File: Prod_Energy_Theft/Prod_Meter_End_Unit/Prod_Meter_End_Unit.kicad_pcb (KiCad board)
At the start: 4 copper layers, 150.7 x 71.9 mm, 83 parts, among them J1 Screw_Terminal_01x02, J15 Screw_Terminal_01x01, J16 Screw_Terminal_01x01, J17 Screw_Terminal_01x01, J18 Screw_Terminal_01x01, J19 Screw_Terminal_01x01, J2 Screw_Terminal_01x02, J20 Screw_Terminal_01x01, J21 Screw_Terminal_01x01, J22 Screw_Terminal_01x01, J23 Screw_Terminal_01x01, J3 Screw_Terminal_01x02, J4 Conn_01x06_Pin, J5 Screw_Terminal_01x02, J6 Jack-DC, K1 TQ2-L2-5V, Q3 AO3400A, Q4 AO3400A, U2 ESP32-C6-MINI-1, U3 BD00FC0WEFJ, U5 ADE7816ACPZ, Y2 Crystal

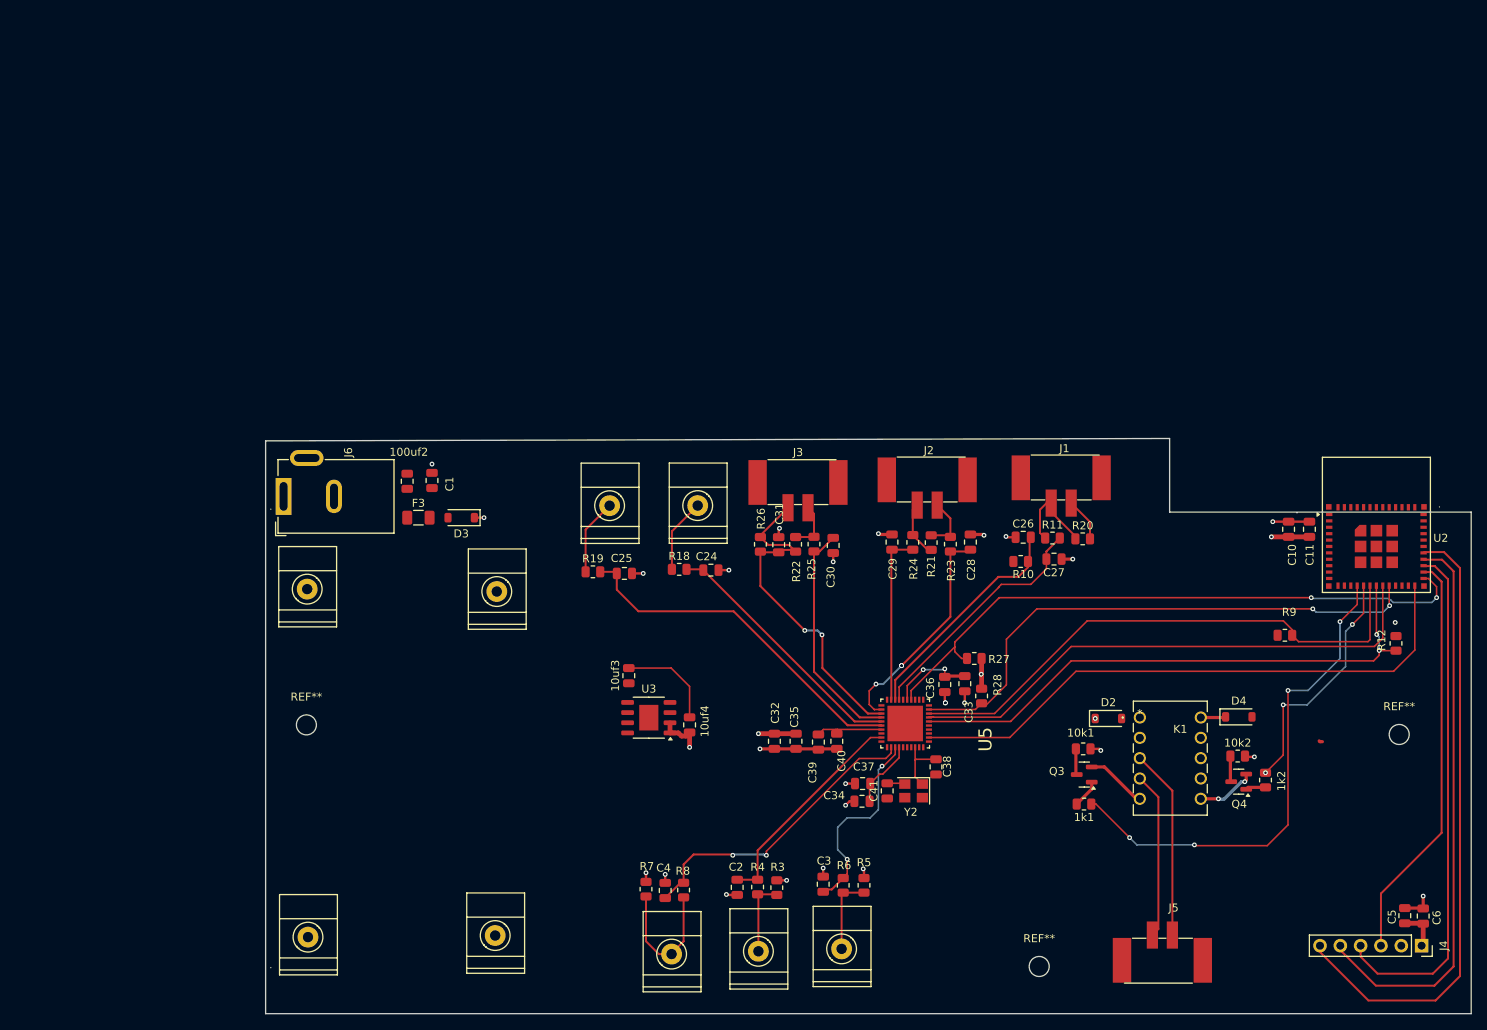
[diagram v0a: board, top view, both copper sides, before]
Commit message: PCB
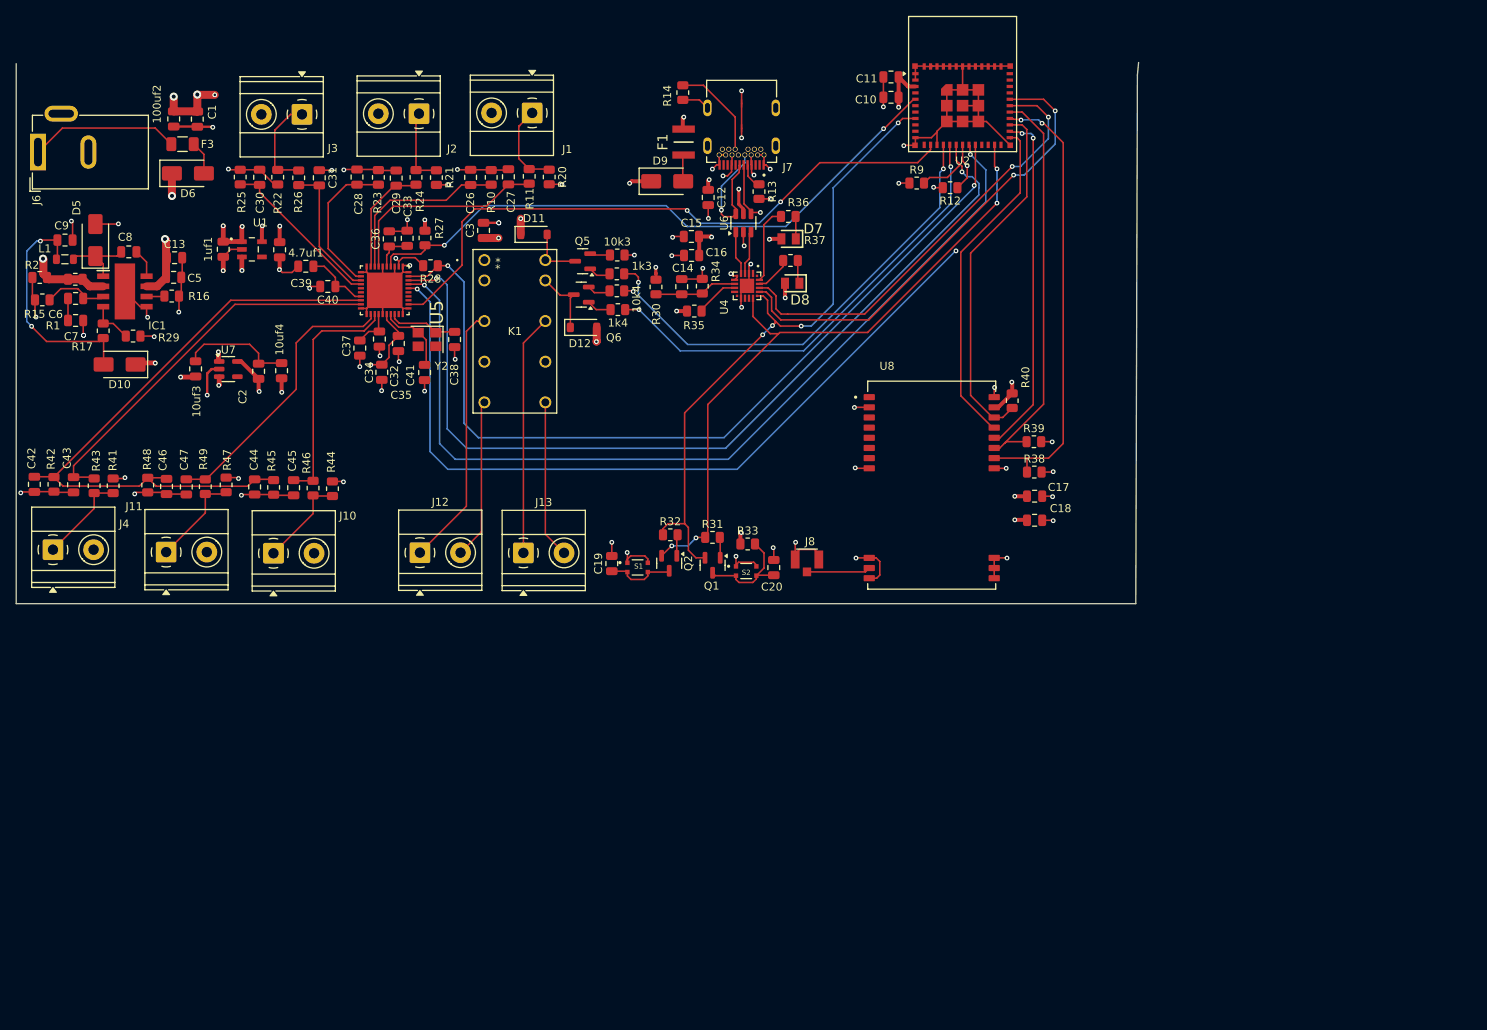
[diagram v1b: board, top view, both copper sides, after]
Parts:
- removed 10k1, 10k2, 1k1, 1k2, R3, R5, R7: R, Resistor_SMD:R_0805_2012Metric
- removed C24, C25, C4: 22nf, Capacitor_SMD:C_0805_2012Metric
- removed D2, D3, D4: D, Diode_SMD:D_SOD-123
- removed J15, J16, J17, J18, J19, J20, J21, J22, J23: Screw_Terminal_01x01, custom:TerminalBlock_1x01_P5.08mm
- removed J5: Screw_Terminal_01x02, TerminalBlock_Phoenix:TerminalBlock_Phoenix_PTSM-0,5-2-2,5-V-SMD_1x02-1MP_P2.50mm_Vertical
- removed Q3, Q4: AO3400A, Package_TO_SOT_SMD:SOT-23
- removed R18, R19: 10k, Resistor_SMD:R_0805_2012Metric
- removed R4, R6, R8: 1k, Resistor_SMD:R_0805_2012Metric
- removed REF** (x3): MountingHole_2.5mm, MountingHole:MountingHole_2.5mm
- removed U3: BD00FC0WEFJ, Package_SO:HTSOP-8-1EP_3.9x4.9mm_P1.27mm_EP2.4x3.2mm
- added 10k3: R, Resistor_SMD:R_0805_2012Metric, F.Cu at (134.8, 67.4)
- added 10k4: R, Resistor_SMD:R_0805_2012Metric, F.Cu at (134.7, 71.8)
- added 1k3: R, Resistor_SMD:R_0805_2012Metric, F.Cu at (134.7, 69.7)
- added 1k4: R, Resistor_SMD:R_0805_2012Metric, F.Cu at (134.8, 74.2)
- added 1uf1: C, Capacitor_SMD:C_0805_2012Metric, F.Cu at (85.5, 66.7)
- added 4.7uf1: C, Capacitor_SMD:C_0805_2012Metric, F.Cu at (92.6, 66.7)
- added C12: 0.1u, Capacitor_SMD:C_0805_2012Metric, F.Cu at (146.1, 60.2)
- added C13: 100nf, Capacitor_SMD:C_0805_2012Metric, F.Cu at (79.4, 67.7)
- added C14: 1u, Capacitor_SMD:C_0805_2012Metric, F.Cu at (142.8, 71.3)
- added C15: 4.7u, Capacitor_SMD:C_0805_2012Metric, F.Cu at (144.0, 65.0)
- added C16: 0.1u, Capacitor_SMD:C_0805_2012Metric, F.Cu at (144.1, 67.4)
- added C17: 10u, Capacitor_SMD:C_0805_2012Metric, F.Cu at (186.9, 97.5)
- added C18: 0.1u, Capacitor_SMD:C_0805_2012Metric, F.Cu at (186.9, 100.5)
- added C19: 0.1u, Capacitor_SMD:C_0805_2012Metric, F.Cu at (134.1, 105.9)
- added C20: 1u, Capacitor_SMD:C_0805_2012Metric, F.Cu at (154.3, 106.4)
- added C42: 22nf, Capacitor_SMD:C_0805_2012Metric, F.Cu at (61.9, 96.0)
- added C43: 22nf, Capacitor_SMD:C_0805_2012Metric, F.Cu at (66.8, 96.1)
- added C44: 22nf, Capacitor_SMD:C_0805_2012Metric, F.Cu at (89.4, 96.4)
- added C45: 22nf, Capacitor_SMD:C_0805_2012Metric, F.Cu at (94.3, 96.5)
- added C46: 22nf, Capacitor_SMD:C_0805_2012Metric, F.Cu at (78.4, 96.3)
- added C47: 22nf, Capacitor_SMD:C_0805_2012Metric, F.Cu at (80.9, 96.3)
- added C7: C, Capacitor_SMD:C_0805_2012Metric, F.Cu at (67.0, 75.5)
- added C8: 100nf, Capacitor_SMD:C_0805_2012Metric, F.Cu at (73.7, 67.0)
- added C9: 47uf, Capacitor_SMD:C_0805_2012Metric, F.Cu at (65.7, 65.5)
- added D10: SS34, Diode_SMD:D_SMA, F.Cu at (72.5, 81.0)
- added D11: D, Diode_SMD:D_SOD-123, F.Cu at (124.3, 64.8)
- added D12: D, Diode_SMD:D_SOD-123, F.Cu at (130.5, 76.4)
- added D5: SS34, Diode_SMD:D_SMA, F.Cu at (69.5, 65.5)
- added D6: SS34, Diode_SMD:D_SMA, F.Cu at (81.1, 57.2)
- added D7: Green, theftdetection:LEDC2012X120N, F.Cu at (156.2, 65.3)
- added D8: Red, theftdetection:LEDC2012X120N, F.Cu at (156.6, 70.9)
- added D9: SS34, Diode_SMD:D_SMA, F.Cu at (141.0, 58.1)
- added F1: 0ZCH0110AF2E, Footprints.kicad_mod:FUSC3226X100N, F.Cu at (143.1, 53.2)
- added IC1: MP1584EN-LF-Z, theftdetection:SOIC127P600X170-9N, F.Cu at (73.2, 71.9)
- added J10: Screw_Terminal_01x02, TerminalBlock_Phoenix:TerminalBlock_Phoenix_MKDS-1,5-2-5.08_1x02_P5.08mm_Horizontal, F.Cu at (91.8, 104.6)
- added J11: Screw_Terminal_01x02, TerminalBlock_Phoenix:TerminalBlock_Phoenix_MKDS-1,5-2-5.08_1x02_P5.08mm_Horizontal, F.Cu at (78.4, 104.5)
- added J12: Screw_Terminal_01x02, TerminalBlock_Phoenix:TerminalBlock_Phoenix_MKDS-1,5-2-5.08_1x02_P5.08mm_Horizontal, F.Cu at (110.1, 104.6)
- added J13: Screw_Terminal_01x02, TerminalBlock_Phoenix:TerminalBlock_Phoenix_MKDS-1,5-2-5.08_1x02_P5.08mm_Horizontal, F.Cu at (123.0, 104.6)
- added J7: SS-52400-002, theftdetection:BELFUSE_SS-52400-002, F.Cu at (150.3, 49.0)
- added J8: U.FL-R-SMT_01_, theftdetection:HRS_U.FL-R-SMT_01_, F.Cu at (158.5, 105.4)
- added L1: 15uH, Inductor_SMD:L_0805_2012Metric, F.Cu at (65.7, 67.9)
- added Q1: BC817, Package_TO_SOT_SMD:SOT-23, F.Cu at (146.7, 106.2)
- added Q2: BC817, Package_TO_SOT_SMD:SOT-23, F.Cu at (141.2, 105.9)
- added Q5: AO3400A, Package_TO_SOT_SMD:SOT-23, F.Cu at (130.4, 68.1)
- added Q6: AO3400A, Package_TO_SOT_SMD:SOT-23, F.Cu at (130.3, 72.3)
- added R1: 100k, Resistor_SMD:R_0805_2012Metric, F.Cu at (67.0, 70.4)
- added R13: 5K1, Resistor_SMD:R_0805_2012Metric, F.Cu at (152.5, 59.4)
- added R14: 5K1, Resistor_SMD:R_0805_2012Metric, F.Cu at (142.9, 47.1)
- added R15: 100k, Resistor_SMD:R_0805_2012Metric, F.Cu at (62.9, 73.0)
- added R16: 100k, Resistor_SMD:R_0805_2012Metric, F.Cu at (79.1, 72.5)
- added R17: 210k, Resistor_SMD:R_0805_2012Metric, F.Cu at (70.5, 76.8)
- added R2: 24k9, Resistor_SMD:R_0805_2012Metric, F.Cu at (62.6, 70.2)
- added R29: 40k2, Resistor_SMD:R_0805_2012Metric, F.Cu at (74.2, 77.5)
- added R30: 20k, Resistor_SMD:R_0805_2012Metric, F.Cu at (139.6, 71.4)
- added R31: 10K, Resistor_SMD:R_0805_2012Metric, F.Cu at (146.7, 102.7)
- added R32: 10K, Resistor_SMD:R_0805_2012Metric, F.Cu at (141.4, 102.3)
- added R33: 10K, Resistor_SMD:R_0805_2012Metric, F.Cu at (151.1, 103.5)
- added R34: 39k, Resistor_SMD:R_0805_2012Metric, F.Cu at (145.4, 71.3)
- added R35: IK, Resistor_SMD:R_0805_2012Metric, F.Cu at (144.4, 74.4)
- added R36: 330, Resistor_SMD:R_0805_2012Metric, F.Cu at (156.1, 62.5)
- added R37: 330, Resistor_SMD:R_0805_2012Metric, F.Cu at (156.4, 68.0)
- added R38: 10k, Resistor_SMD:R_0805_2012Metric, F.Cu at (186.9, 94.5)
- added R39: 10k, Resistor_SMD:R_0805_2012Metric, F.Cu at (186.8, 90.7)
- added R40: 10k, Resistor_SMD:R_0805_2012Metric, F.Cu at (184.1, 85.6)
- added R41: 10, Resistor_SMD:R_0805_2012Metric, F.Cu at (71.7, 96.2)
- added R42: 1K, Resistor_SMD:R_0805_2012Metric, F.Cu at (64.3, 96.0)
- added R43: 1K, Resistor_SMD:R_0805_2012Metric, F.Cu at (69.4, 96.2)
- added R44: 10, Resistor_SMD:R_0805_2012Metric, F.Cu at (99.2, 96.6)
- added R45: 1K, Resistor_SMD:R_0805_2012Metric, F.Cu at (91.8, 96.4)
- added R46: 1K, Resistor_SMD:R_0805_2012Metric, F.Cu at (96.7, 96.5)
- added R47: 10, Resistor_SMD:R_0805_2012Metric, F.Cu at (85.9, 96.1)
- added R48: 1K, Resistor_SMD:R_0805_2012Metric, F.Cu at (76.1, 96.1)
- added R49: 1K, Resistor_SMD:R_0805_2012Metric, F.Cu at (83.3, 96.3)
- added S1: BOOT, theftdetection:SW_USLPT2819DT2TR, F.Cu at (137.3, 106.4)
- added S2: RESET, theftdetection:SW_USLPT2819DT2TR, F.Cu at (150.9, 106.9)
- added U1: TPS7A2033PDBVR, theftdetection:SOT95P280X145-5N, F.Cu at (89.1, 66.7)
- added U4: CP2102N-Axx-xQFN20, theftdetection:IC_CP2102N-A01-GQFN20, F.Cu at (151.0, 71.2)
- added U6: USBLC6-2SC6, Package_TO_SOT_SMD:SOT-23-6, F.Cu at (150.5, 63.4)
- added U7: AP2112K-3.3, Package_TO_SOT_SMD:SOT-23-5, F.Cu at (86.1, 81.6)
- added U8: E32-433T20S, theftdetection:MODULE_E32-433T20S, F.Cu at (174.1, 96.1)
- C2: value 22nf -> 100nf
- C3: value 22nf -> 100uf
- C5: value 10u -> 10uf
- C6: value 0.1u -> 150pf
- J1, J2, J3: footprint TerminalBlock_Phoenix:TerminalBlock_Phoenix_PTSM-0,5-2-2,5-V-SMD_1x02-1MP_P2.50mm_Vertical -> TerminalBlock_Phoenix:TerminalBlock_Phoenix_MKDS-1,5-2-5.08_1x02_P5.08mm_Horizontal
- J4: value Conn_01x06_Pin -> Screw_Terminal_01x02; footprint Connector_PinSocket_2.54mm:PinSocket_1x06_P2.54mm_Vertical -> TerminalBlock_Phoenix:TerminalBlock_Phoenix_MKDS-1,5-2-5.08_1x02_P5.08mm_Horizontal
- K1: value TQ2-L2-5V -> HFD2/012-S-L2-D; footprint footprints:RELAY_TQ2_2C_PAN -> theftdetection:RELAY10_HFD2&slash_012_HNG
- moved C6 185.3 mm to (67.0, 72.8), turned to 180 degrees
- moved J4 178.1 mm to (64.2, 104.2), turned to 0 degrees
- moved C5 173.3 mm to (79.3, 70.2), turned to 0 degrees
- moved K1 99.9 mm to (118.1, 68.0)
- moved C3 92.1 mm to (118.0, 64.3)
- moved C28 89.2 mm to (102.2, 57.6)
- moved C33 89.2 mm to (108.5, 65.3), turned to -90 degrees
- moved C36 89.0 mm to (106.2, 65.3), turned to 90 degrees
- moved C2 88.0 mm to (89.9, 81.9), turned to 90 degrees
- moved C39 87.4 mm to (95.8, 68.8), turned to 180 degrees
- moved R28 87.4 mm to (111.4, 68.7), turned to 180 degrees
- moved R27 86.5 mm to (110.7, 65.2), turned to -90 degrees
- moved C40 85.3 mm to (98.6, 71.3), turned to 180 degrees
- moved C30 85.2 mm to (90.0, 57.6), turned to -90 degrees
- moved R25 85.1 mm to (87.6, 57.6)
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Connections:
- net Net-(U5-CLKIN) renamed /ESP32/ADE7816/CLKIN
- net Net-(U5-IAN) renamed /ESP32/ADE7816/IAN
- net Net-(U5-IAP) renamed /ESP32/ADE7816/IAP
- net Net-(U5-IBN) renamed /ESP32/ADE7816/IBN
- net Net-(U5-IBP) renamed /ESP32/ADE7816/IBP
- net Net-(U5-ICN) renamed /ESP32/ADE7816/ICN
- net Net-(U5-ICP) renamed /ESP32/ADE7816/ICP
- C2 pad 1: Net-(U5-IFP) -> +3.3V
- C2 pad 2: GND -> Net-(10uf3-Pad2)
- C3 pad 1: Net-(U5-IDP) -> +12V
- C32 pad 1: +3.3V -> +3.3V_ADE
- C35 pad 1: +3.3V -> +3.3V_ADE
- C5 pad 1: +3.3V -> +12V
- C6 pad 1: +3.3V -> Net-(IC1-COMP)
- C6 pad 2: GND -> Net-(C6-Pad2)
- J1 pad 2: Net-(J1-Pin_2) -> GND
- J2 pad 2: Net-(J2-Pin_2) -> GND
- J3 pad 2: Net-(J3-Pin_2) -> GND
- J4 pad 1: +3.3V -> Net-(J4-Pin_1)
- K1 pad 1: Net-(D2-A) -> +12V
- K1 pad 2: unconnected-(K1-Pad2) -> +12V
- K1 pad 6: Net-(Q4-S) -> unconnected-(K1-Pad6)
- K1 pad 8: unconnected-(K1-Pad8) -> Net-(J12-Pin_2)
- K1 pad 9: unconnected-(K1-Pad9) -> Net-(J13-Pin_2)
- R10 pad 1: Net-(J1-Pin_2) -> GND
- R20 pad 2: Net-(J1-Pin_2) -> GND
- R21 pad 2: Net-(J2-Pin_2) -> GND
- R22 pad 2: Net-(J3-Pin_2) -> GND
- R23 pad 1: Net-(J2-Pin_2) -> GND
- R25 pad 1: Net-(J3-Pin_2) -> GND
- R27 pad 1: +3.3V -> +3.3V_ADE
- R28 pad 2: +3.3V -> +3.3V_ADE
- U2 pad 13: unconnected-(U2-IO1-Pad13) -> /ESP32/IRQ
- U2 pad 15: /ESP32/MCB_CTRL -> /ESP32/MCB_SET
- U2 pad 16: /ESP32/MCB_CTRL_D -> /ESP32/MCB_RESET
- U2 pad 23: unconnected-(U2-IO9-Pad23) -> /ESP32/DTR
- U2 pad 24: /ESP32/IRQ -> unconnected-(U2-IO18-Pad24)
- U2 pad 25: /ESP32/RES -> /ESP32/LORA_TX
- U2 pad 26: /ESP32/LORA_TX -> /ESP32/LORA_RX
- U2 pad 27: /ESP32/LORA_RX -> /ESP32/LORA_AUX
- U2 pad 28: /ESP32/LORA_AUX -> /ESP32/LORA_MD0
- U2 pad 29: /ESP32/LORA_MD0 -> /ESP32/LORA_MD1
- U2 pad 30: unconnected-(U2-RXD0-Pad30) -> /ESP32/TX_RX
- U2 pad 31: unconnected-(U2-TXD0-Pad31) -> /ESP32/RX_TX
- U2 pad 5: unconnected-(U2-IO2-Pad5) -> /ESP32/RES
- U2 pad 8: unconnected-(U2-EN-Pad8) -> /ESP32/RTS
- U5 pad 15: Net-(U5-VP) -> unconnected-(U5-VP-Pad15)
- U5 pad 16: Net-(U5-VN) -> unconnected-(U5-VN-Pad16)
- U5 pad 18: GND -> /ESP32/ADE7816/IN
- U5 pad 19: Net-(U5-IFP) -> /ESP32/ADE7816/IFP
- U5 pad 2: +3.3V -> +3.3V_ADE
- U5 pad 22: Net-(U5-IEP) -> /ESP32/ADE7816/IEP
- U5 pad 23: Net-(U5-IDP) -> /ESP32/ADE7816/IDP
- U5 pad 26: +3.3V -> +3.3V_ADE
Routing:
- net GND: track 44.0 -> 268.1 mm, vias 25 -> 66
- net /ESP32/DTR: track 0.00 -> 83.5 mm, vias 0 -> 4
- net /ESP32/ADE7816/IN: track 0.00 -> 81.6 mm
- net /ESP32/RTS: track 0.00 -> 81.4 mm, vias 0 -> 4
- net +3.3V: track 24.5 -> 97.7 mm, vias 4 -> 14
- net +5V: track 150.9 -> 79.5 mm, vias 1 -> 8
- net /ESP32/MCB_CTRL: track 62.8 -> 0.00 mm, vias 4 -> 0
- net /ESP32/MCB_SET: track 0.00 -> 59.6 mm, vias 0 -> 2
- net /ESP32/RX_TX: track 0.00 -> 58.9 mm, vias 0 -> 2
- net /ESP32/MCB_RESET: track 0.00 -> 58.1 mm, vias 0 -> 2
- net /ESP32/TX_RX: track 0.00 -> 55.6 mm, vias 0 -> 2
- net /ESP32/LORA_MD1: track 0.00 -> 50.6 mm
- net /ESP32/SCLK/SCL: track 68.3 -> 117.3 mm, vias 0 -> 2
- net /ESP32/ADE7816/IFP: track 0.00 -> 48.3 mm
- net /ESP32/MOSI/SDA: track 70.7 -> 117.5 mm, vias 2 -> 3
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- added copper zone on In2.Cu, net +3.3V_ADE
- added copper zone on In2.Cu, net +5V
- added copper zone on In2.Cu, net /VBUS
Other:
- board size 150.7 x 71.9 mm -> 140.3 x 67.7 mm
